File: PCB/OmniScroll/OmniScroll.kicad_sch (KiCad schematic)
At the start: 47 parts, among them J1 Conn_01x02_Pin, J2 Conn_01x01_Pin, J3 Conn_01x01_Pin, J4 Conn_01x01_Pin, J5 Conn_01x01_Pin, J6 UJC-H-G-SMT-P6-TR, Q1 BSS138, Q2 BSS138, SW1 SW_DIP_x01, U1 MCP73831-2-OT, U2 nRF52840_holyiot_18010, U3 TMAG5273A1QDBVT, U4 TPS7A0233PDBVR

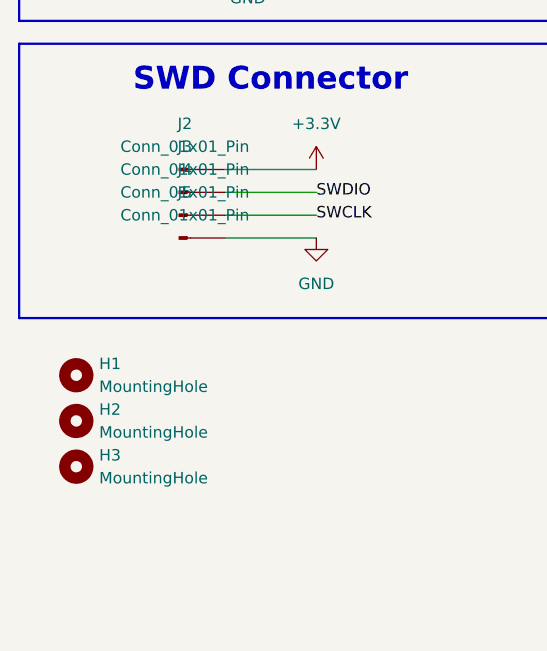
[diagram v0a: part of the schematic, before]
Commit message: V1.1
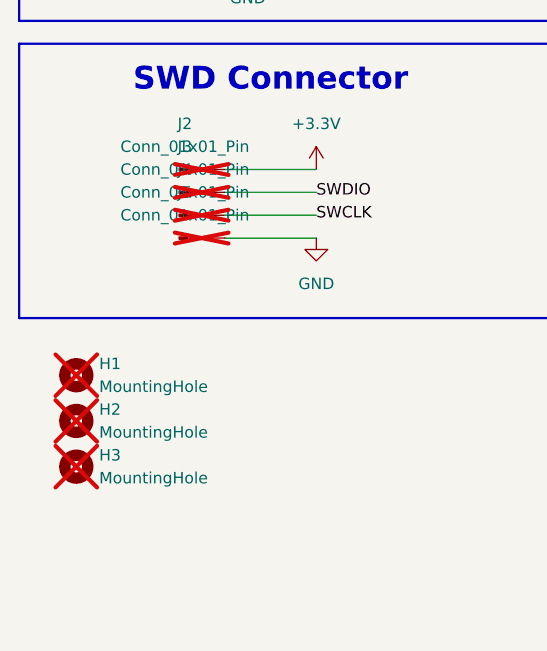
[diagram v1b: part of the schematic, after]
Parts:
- C1, C3: Manufacturer_Part_Number (none) -> GRT188C81C475KE13D
- C2, C4, C5, C6: Manufacturer_Part_Number (none) -> GRM188R61C105KA12J
- D1, D3, D4: Manufacturer_Part_Number (none) -> LTST-C190KRKT
- D2: Manufacturer_Part_Number (none) -> LTST-C190GKT
- D5: Manufacturer_Part_Number (none) -> 150060BS75000
- F1: Manufacturer_Part_Number (none) -> FCC16201ABTP
- H1, H2, H3: now not fitted
- J1: Manufacturer_Part_Number (none) -> 53048-0210
- J2, J3, J4, J5: now not fitted; now left out of the parts list
- Q1, Q2: Manufacturer_Part_Number (none) -> BSS138
- R1, R2: Manufacturer_Part_Number (none) -> RC0603FR-075K1P
- R10, R16, R17, R18: Manufacturer_Part_Number (none) -> CRGCQ0603F100K
- R11, R12, R13, R14, R15, R19, R4, R5, R6, R7: Manufacturer_Part_Number (none) -> AC0603JR-131KL
- R3: Manufacturer_Part_Number (none) -> RMCA0603FT20K0-HP
- R9: Manufacturer_Part_Number (none) -> RMCA0603JT10K0-HP
- SW1: Manufacturer_Part_Number (none) -> DM-01-V
- U1: Manufacturer_Part_Number (none) -> MCP73831T-2ACI/OT
- U2: now left out of the parts list
- U3: Manufacturer_Part_Number (none) -> TMAG5273C1QDBVR
- U4: Manufacturer_Part_Number (none) -> TPS7A0233PDBVR
